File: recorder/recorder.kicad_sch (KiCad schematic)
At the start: 2 parts, among them U1 IM73D122V01, U2 ADAU7118

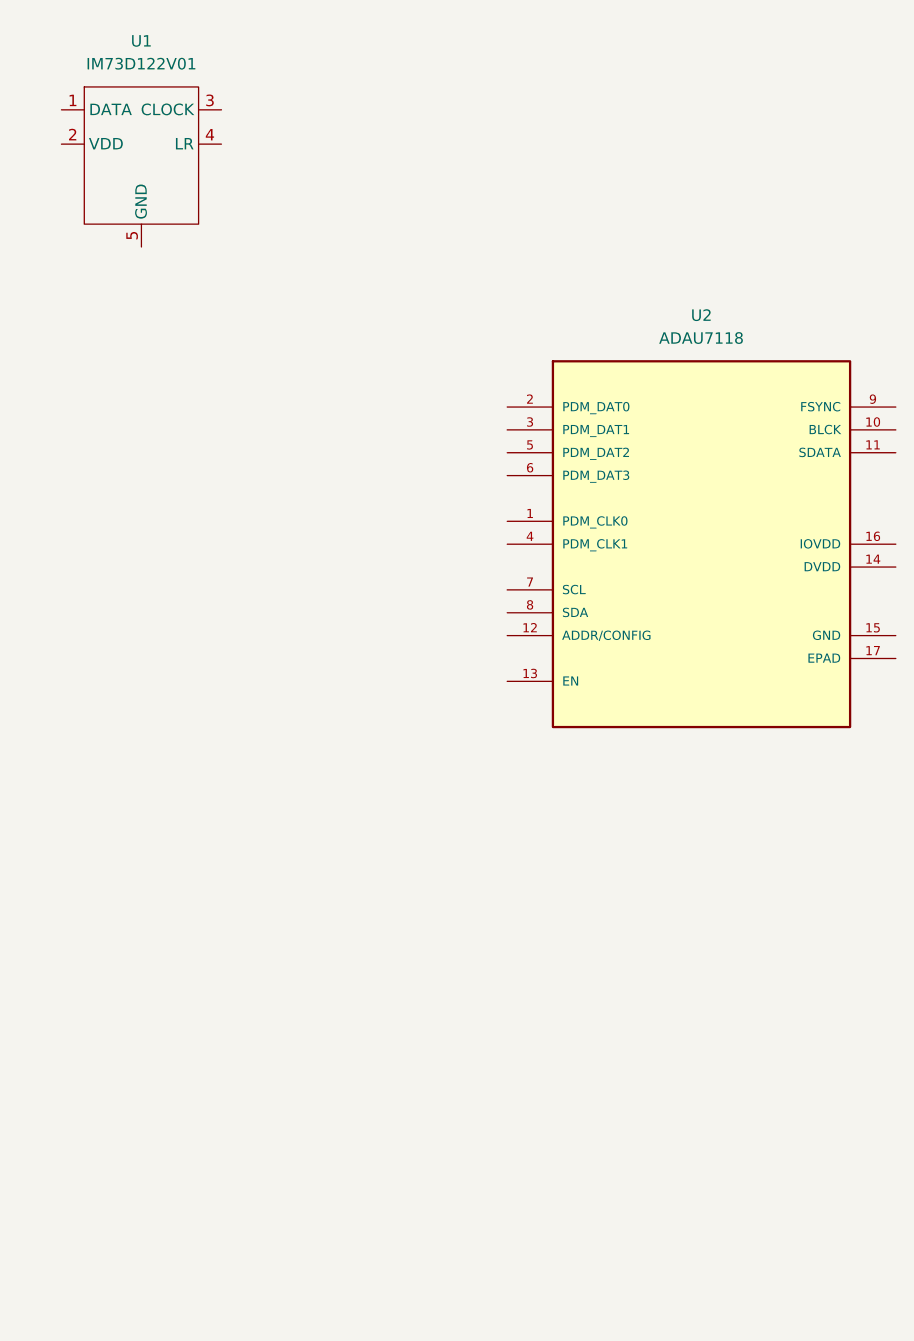
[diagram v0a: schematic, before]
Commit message: schematics start
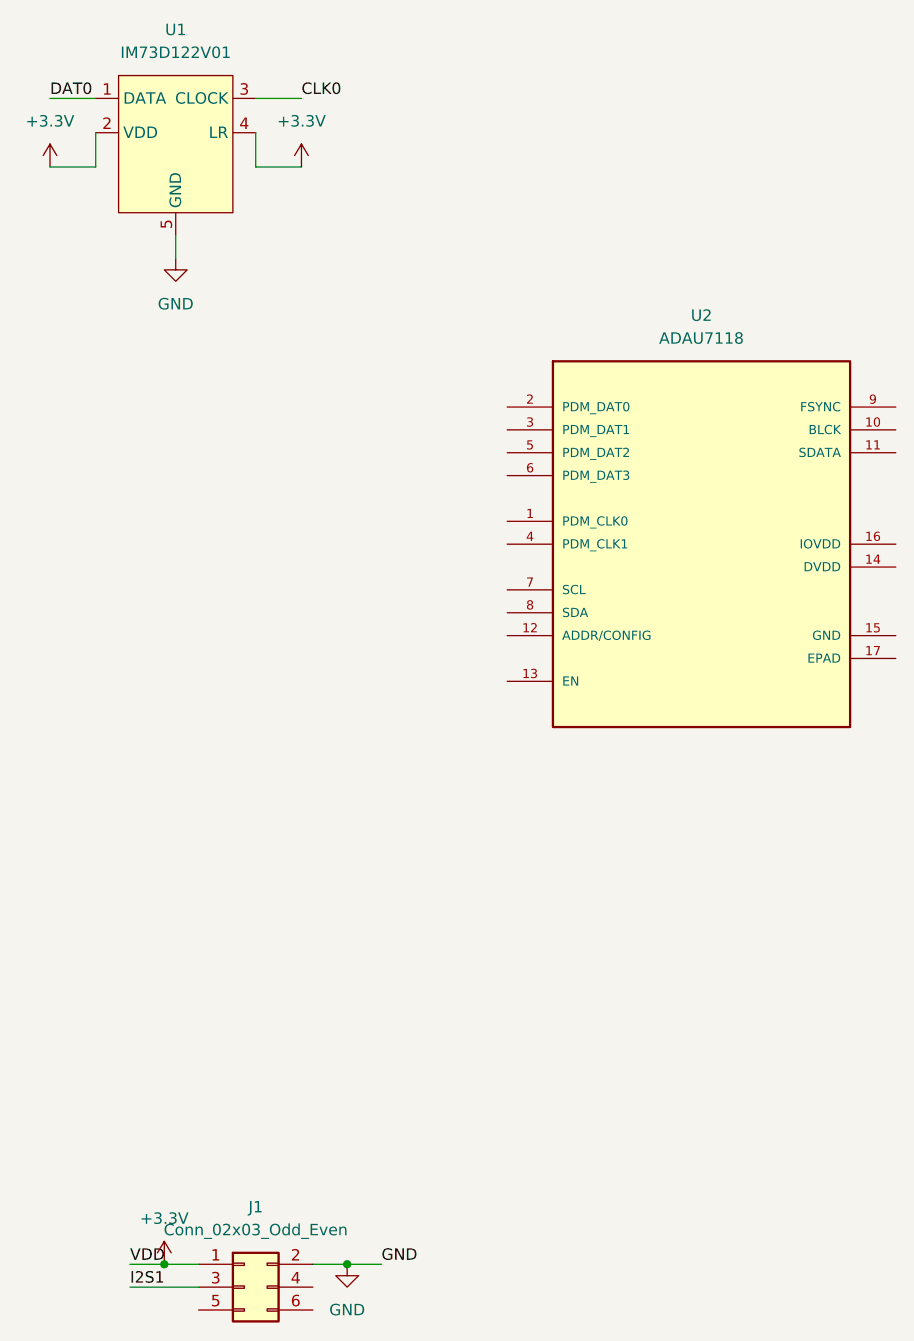
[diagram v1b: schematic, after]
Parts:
- added J1: Conn_02x03_Odd_Even, symbol recorder:JETSON_CONNECTOR
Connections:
- net DAT0: now reaches U1.1 (DATA)
- net +3.3V: now reaches U1.2 (VDD)
- net +3.3V: now also U1.4 (LR), J1.1 (Vcc)
- net CLK0: now reaches U1.3 (CLOCK)
- net GND: now reaches U1.5 (GND)
- net GND: now also J1.2 (GND)
- new net I2S1: J1.3 (I2S1)
